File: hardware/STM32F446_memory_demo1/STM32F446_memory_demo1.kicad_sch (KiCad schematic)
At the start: 0 parts

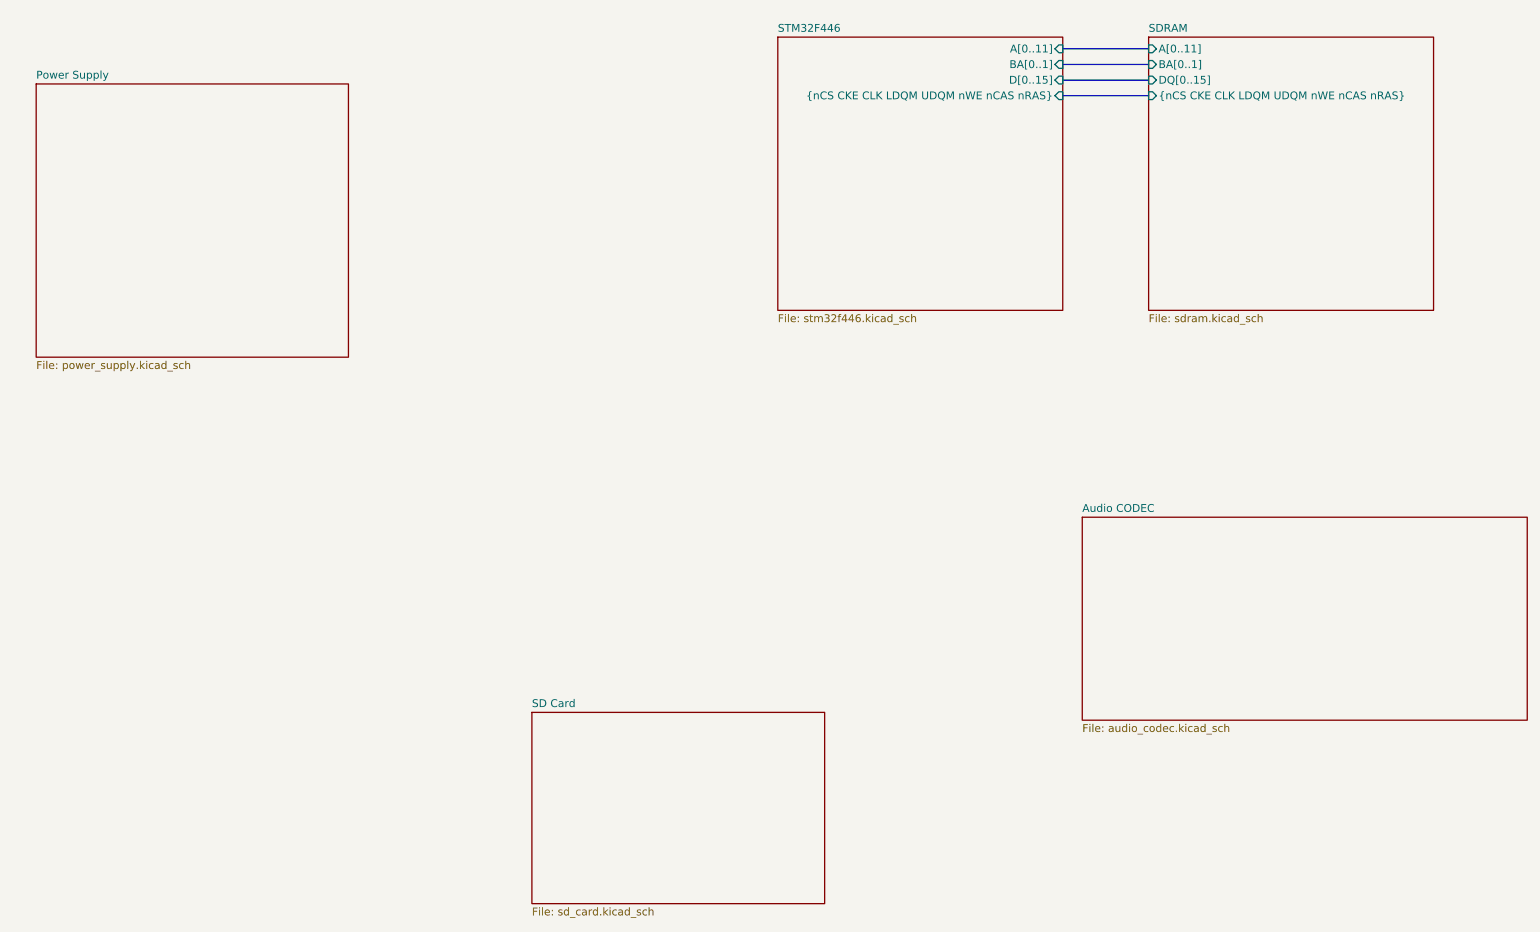
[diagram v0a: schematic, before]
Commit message: some schematics
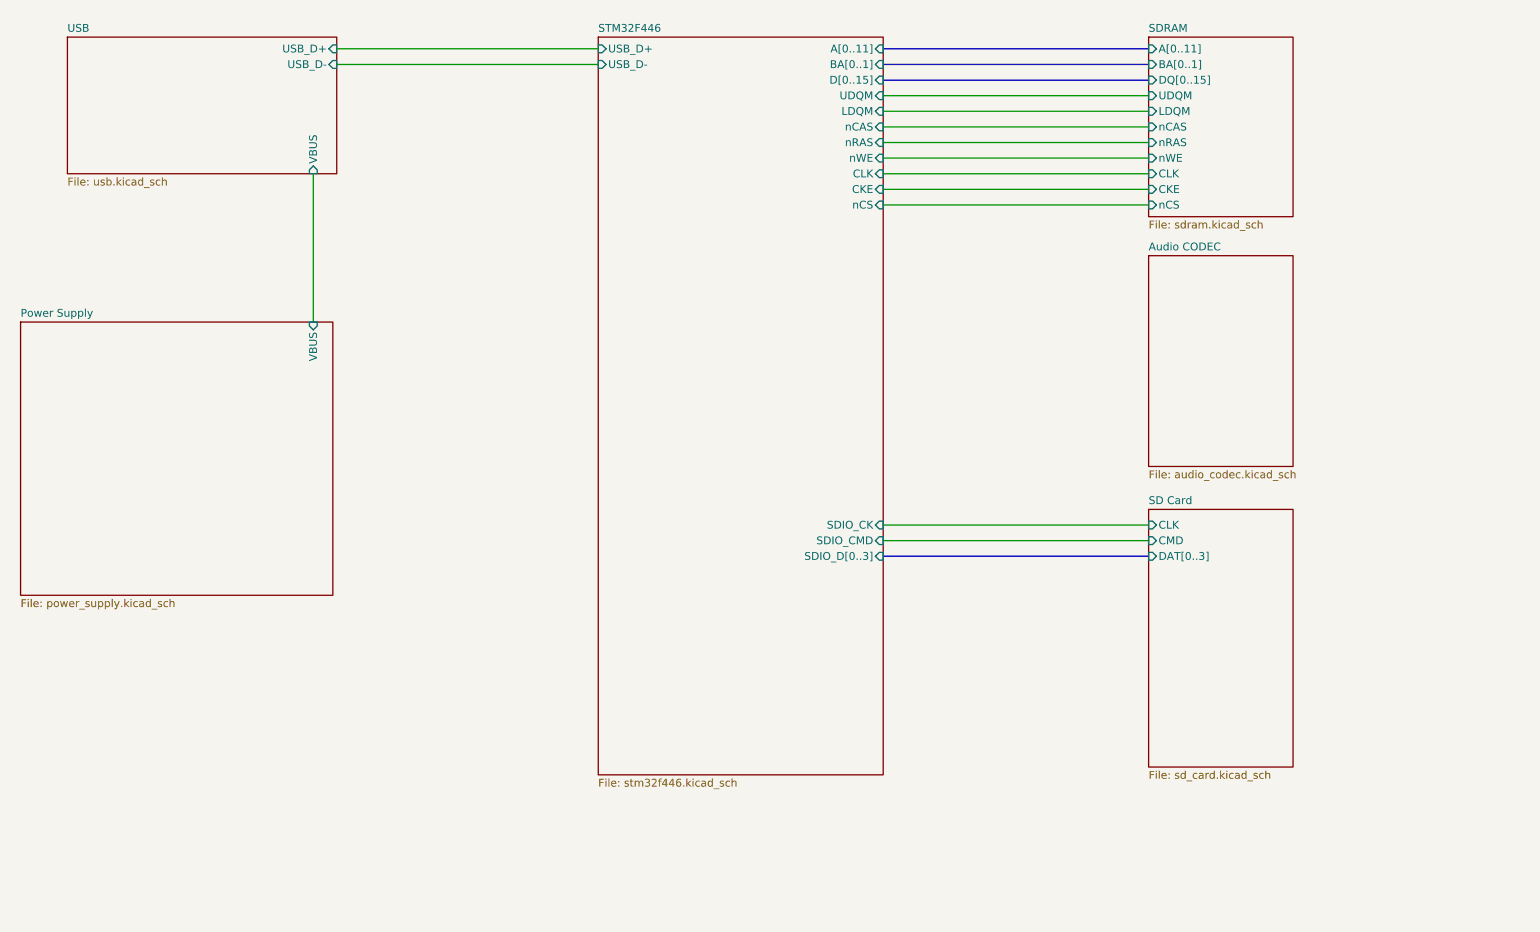
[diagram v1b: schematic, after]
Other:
- added sheet USB (usb.kicad_sch)
- sheet Power Supply ports: added VBUS; removed none
- sheet SD Card ports: added CLK, CMD, DAT[0..3]; removed none
- sheet SDRAM ports: added CKE, CLK, LDQM, UDQM, nCAS, nCS, nRAS, nWE; removed {nCS CKE CLK LDQM UDQM nWE nCAS nRAS}
- sheet STM32F446 ports: added CKE, CLK, LDQM, SDIO_CK, SDIO_CMD, SDIO_D[0..3], UDQM, USB_D+, USB_D-, nCAS, nCS, nRAS, nWE; removed {nCS CKE CLK LDQM UDQM nWE nCAS nRAS}

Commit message: added a lot of stuff a long time ago :S
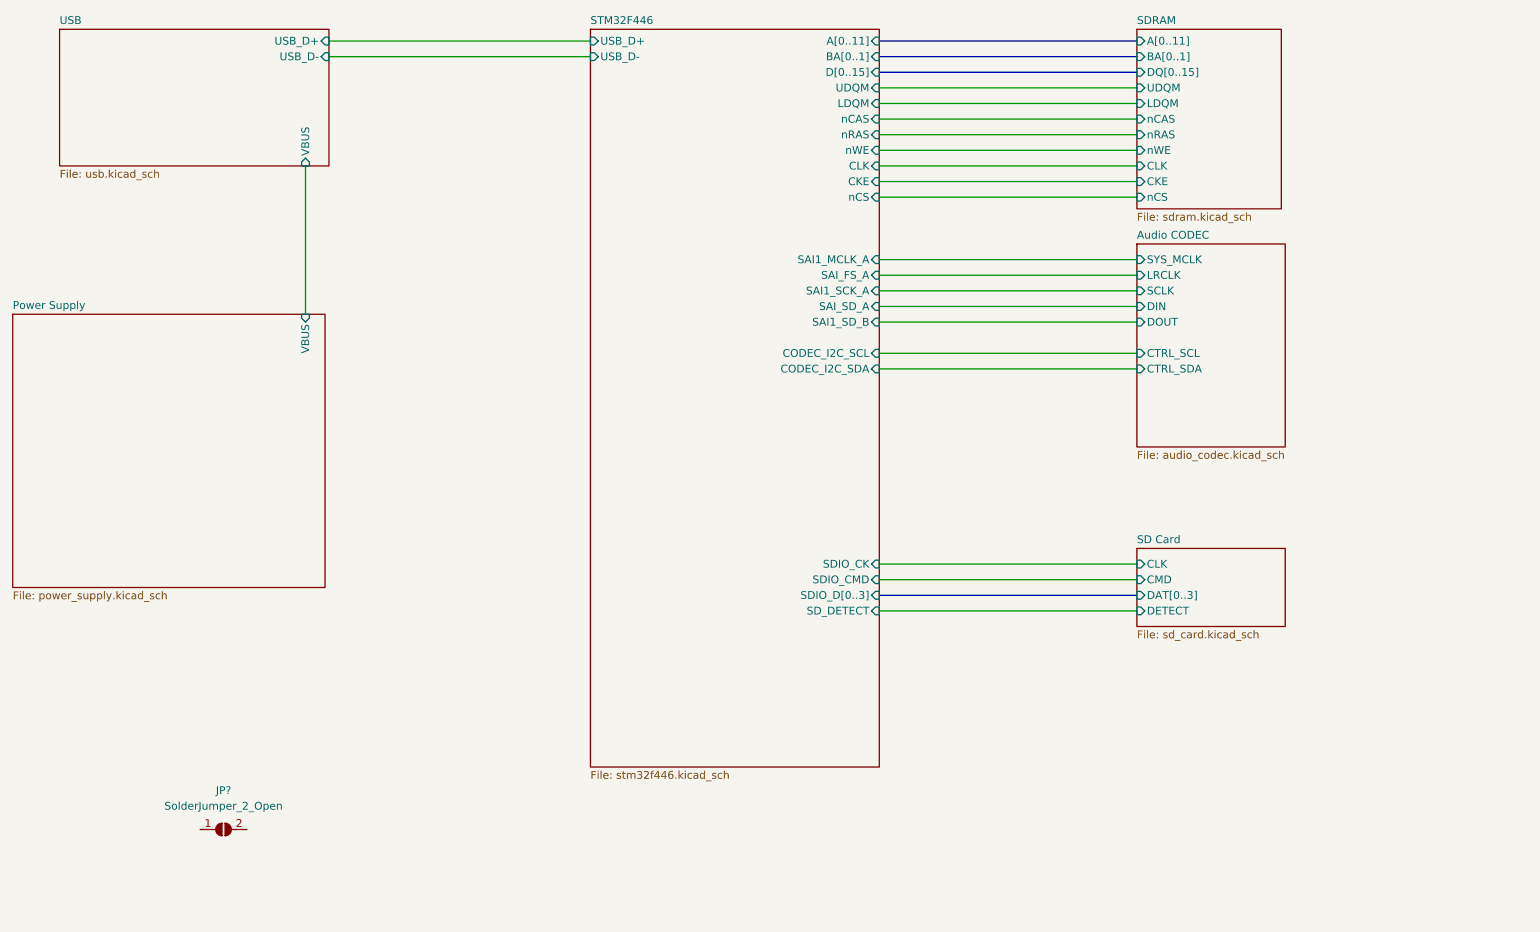
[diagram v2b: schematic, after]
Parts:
- added JP?: SolderJumper_2_Open, symbol Jumper:SolderJumper_2_Open
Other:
- sheet Audio CODEC ports: added CTRL_SCL, CTRL_SDA, DIN, DOUT, LRCLK, SCLK, SYS_MCLK; removed none
- sheet SD Card ports: added DETECT; removed none
- sheet STM32F446 ports: added CODEC_I2C_SCL, CODEC_I2C_SDA, SAI1_MCLK_A, SAI1_SCK_A, SAI1_SD_B, SAI_FS_A, SAI_SD_A, SD_DETECT; removed none
